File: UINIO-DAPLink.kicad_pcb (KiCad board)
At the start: 2 copper layers, 94.1 x 30 mm, 51 parts, among them J1 扩展板串口 & 电源输出, J2 扩展板 JTAG 输出, J3 JTAG_nTRST 跳线选择, J4 3.3V 跳线选择, J5 扩展板 SWD 输入, J6 DAPLink 固件下载接口, J7 SWD 下载输出, U1 ME6211C33M5G, U2 STM32F103C8T6, Y1 8MHz

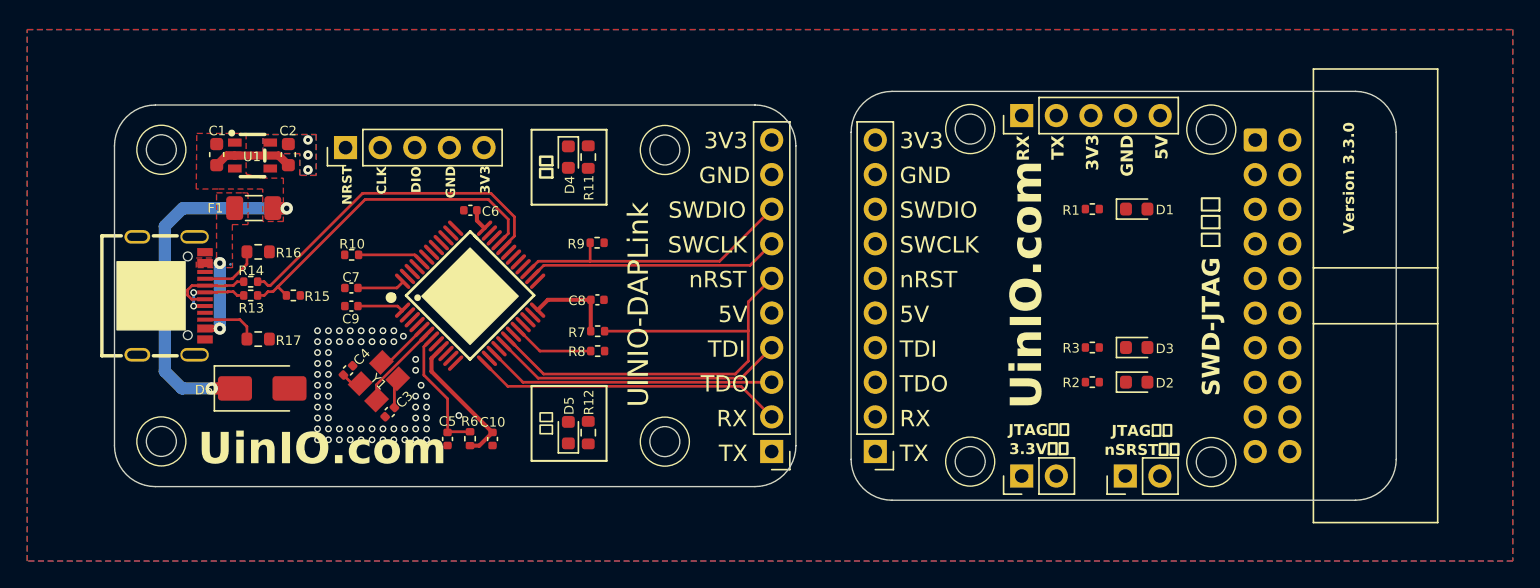
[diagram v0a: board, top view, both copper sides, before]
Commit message: Finish PCB Layout.
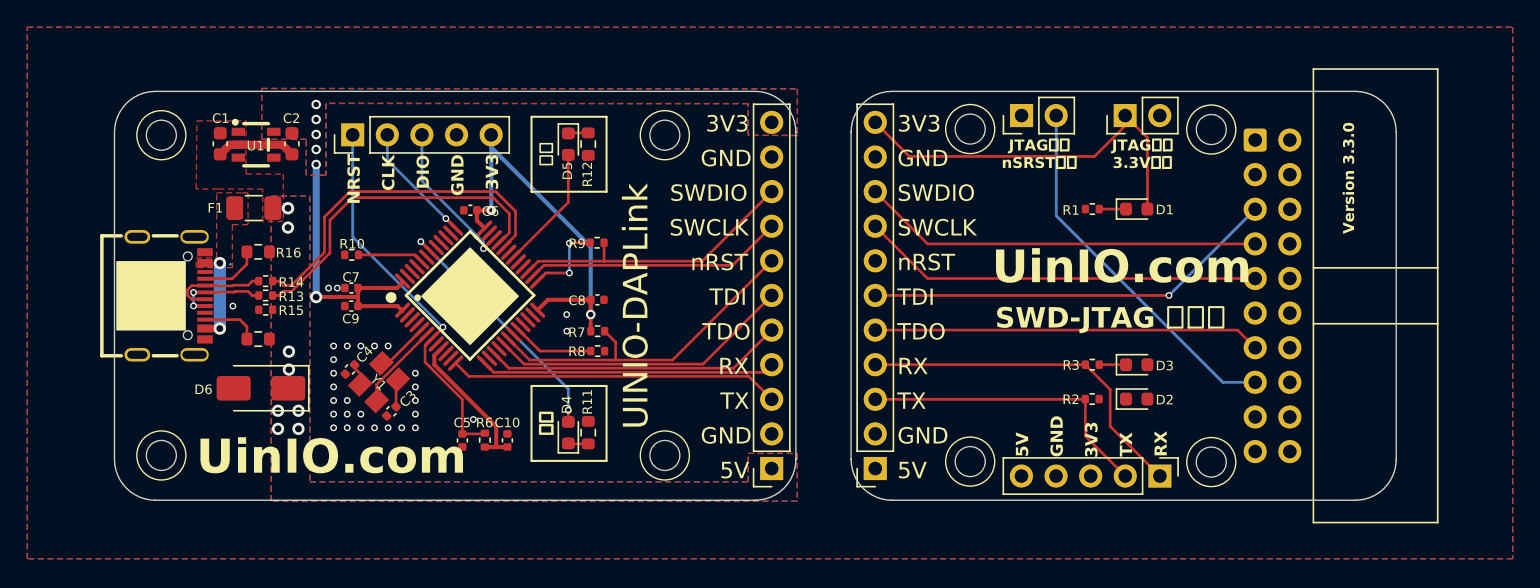
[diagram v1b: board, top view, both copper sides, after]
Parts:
- J5, J7: footprint Connector_PinHeader_2.54mm:PinHeader_1x10_P2.54mm_Vertical -> Connector_PinSocket_2.54mm:PinSocket_1x11_P2.54mm_Vertical
- moved J1 28.3 mm to (176.0, 115.9), turned to -90 degrees
- moved J3 27.5 mm to (165.9, 89.4)
- moved J4 27.5 mm to (173.5, 89.4)
- moved D5 21.2 mm to (132.6, 91.5), turned to -90 degrees
- moved R12 21.2 mm to (134.1, 91.5), turned to -90 degrees
- moved D4 20.2 mm to (132.6, 112.7), turned to 90 degrees
- moved R11 20.2 mm to (134.1, 112.7), turned to 90 degrees
- moved R15 2.29 mm to (110.4, 103.7)
- moved D3 1.26 mm to (174.3, 107.7)
- moved R3 1.26 mm to (171.1, 107.7)
- moved J5 1.25 mm to (155.1, 115.3)
- moved J7 1.25 mm to (147.5, 115.3)
- moved R2 1.24 mm to (171.1, 110.2)
- moved D2 1.24 mm to (174.3, 110.2)
- moved R14 1.10 mm to (110.4, 101.6)
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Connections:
- J5 pad 1: /_USART2_TX -> /_VDD_5V_Fuse
- J5 pad 10: /_VDD_3.3V -> GND
- J5 pad 2: /_USART2_RX -> GND
- J5 pad 3: /_JTAG_TDO -> /_USART2_TX
- J5 pad 4: /_JTAG_TDI -> /_USART2_RX
- J5 pad 5: /_VDD_5V_Fuse -> /_JTAG_TDO
- J5 pad 6: /_JTAG_nRST -> /_JTAG_TDI
- J5 pad 7: /_JTAG_TCK/SWCLK -> /_JTAG_nRST
- J5 pad 8: /_JTAG_TMS/SWDIO -> /_JTAG_TCK/SWCLK
- J5 pad 9: GND -> /_JTAG_TMS/SWDIO
- J7 pad 1: /USART2_TX -> /VDD_5V_Fuse
- J7 pad 10: /VDD_3.3V -> GND
- J7 pad 2: /USART2_RX -> GND
- J7 pad 3: /JTAG_TDO -> /USART2_TX
- J7 pad 4: /JTAG_TDI -> /USART2_RX
- J7 pad 5: /VDD_5V_Fuse -> /JTAG_TDO
- J7 pad 6: /JTAG_nRST -> /JTAG_TDI
- J7 pad 7: /JTAG_TCK/SWCLK -> /JTAG_nRST
- J7 pad 8: /JTAG_TMS/SWDIO -> /JTAG_TCK/SWCLK
- J7 pad 9: GND -> /JTAG_TMS/SWDIO
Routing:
- net /VDD_3.3V: track 25.4 -> 62.3 mm, vias 3 -> 8
- net /_JTAG_TDI: track 0.00 -> 30.5 mm, vias 0 -> 1
- net /_JTAG_TMS/SWDIO: track 0.00 -> 29.5 mm
- net /_JTAG_TCK/SWCLK: track 0.00 -> 29.5 mm
- net /_JTAG_TDO: track 0.00 -> 28.4 mm
- net /_VDD_3.3V: track 0.00 -> 27.8 mm
- net /_JTAG_nRST_Output: track 0.00 -> 27.0 mm
- net /VDD_5V_Fuse: track 26.9 -> 0.04 mm, vias 2 -> 8
- net /_USART2_RX: track 0.00 -> 25.9 mm
- net /USART2_TX: track 0.00 -> 24.3 mm
- net /_USART2_TX: track 0.00 -> 22.2 mm
- net Net-(D4-A): track 0.00 -> 18.8 mm, vias 0 -> 2
- net /NRST: track 9.48 -> 27.7 mm, vias 0 -> 1
- net /Download_SWDIO: track 0.00 -> 11.1 mm, vias 0 -> 1
- net /JTAG_nRST: track 36.4 -> 25.4 mm
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- added copper zone on B.Cu, net /VDD_5V_Fuse
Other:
- outline, holes or cut-outs redrawn
- board text added: "JTAG接口 3.3V跳线"
- board text added: "JTAG接口 nSRST跳线"
- board text removed: "3.3V跳线"
- board text removed: "JTAG接口"
- board text removed: "nSRST跳线"
